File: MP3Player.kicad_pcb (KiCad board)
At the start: 4 copper layers, 40 x 60 mm, 8 parts, among them J1 3.5mm TRRS, SW1 Switch_Tactile_ESwitch, SW2 Switch_Tactile_ESwitch, SW3 Switch_Tactile_ESwitch, SW4 Switch_Tactile_ESwitch, U1 DFR0299, U2 DM-OLED096-636

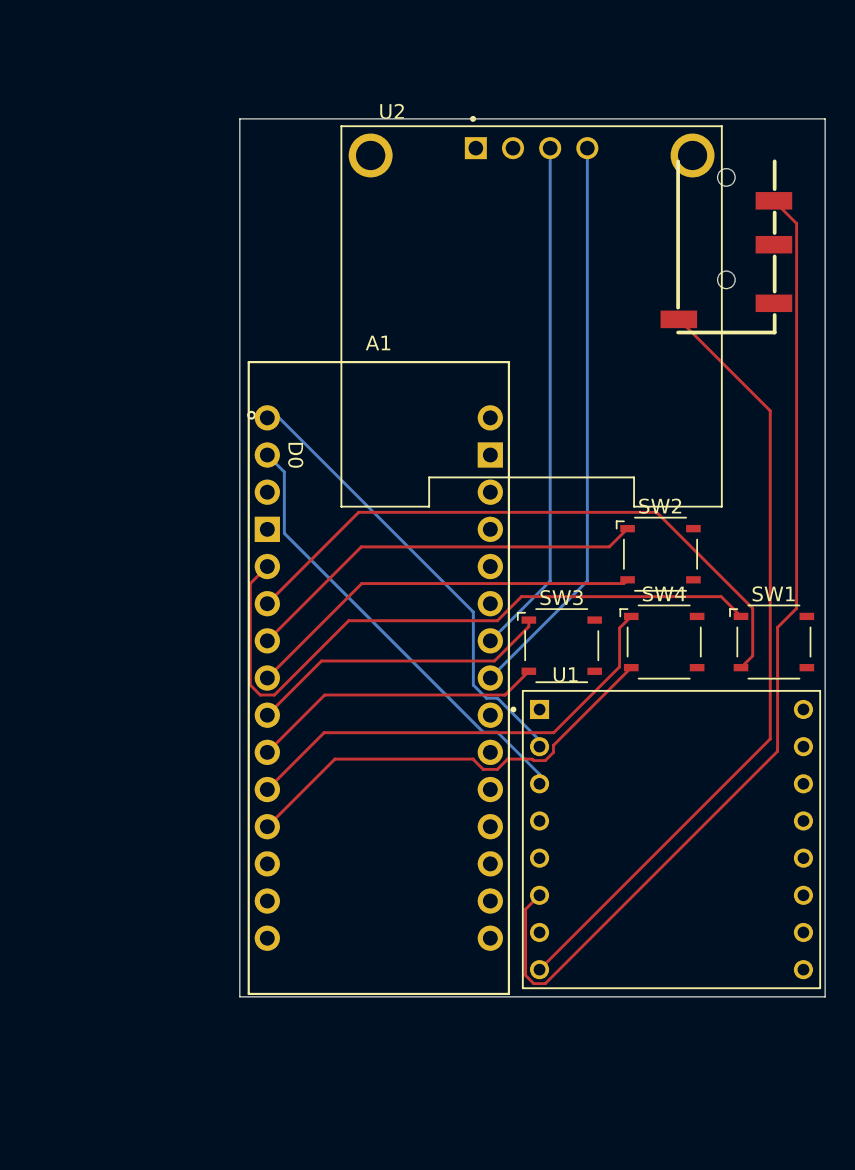
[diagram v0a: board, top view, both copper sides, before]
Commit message: general update
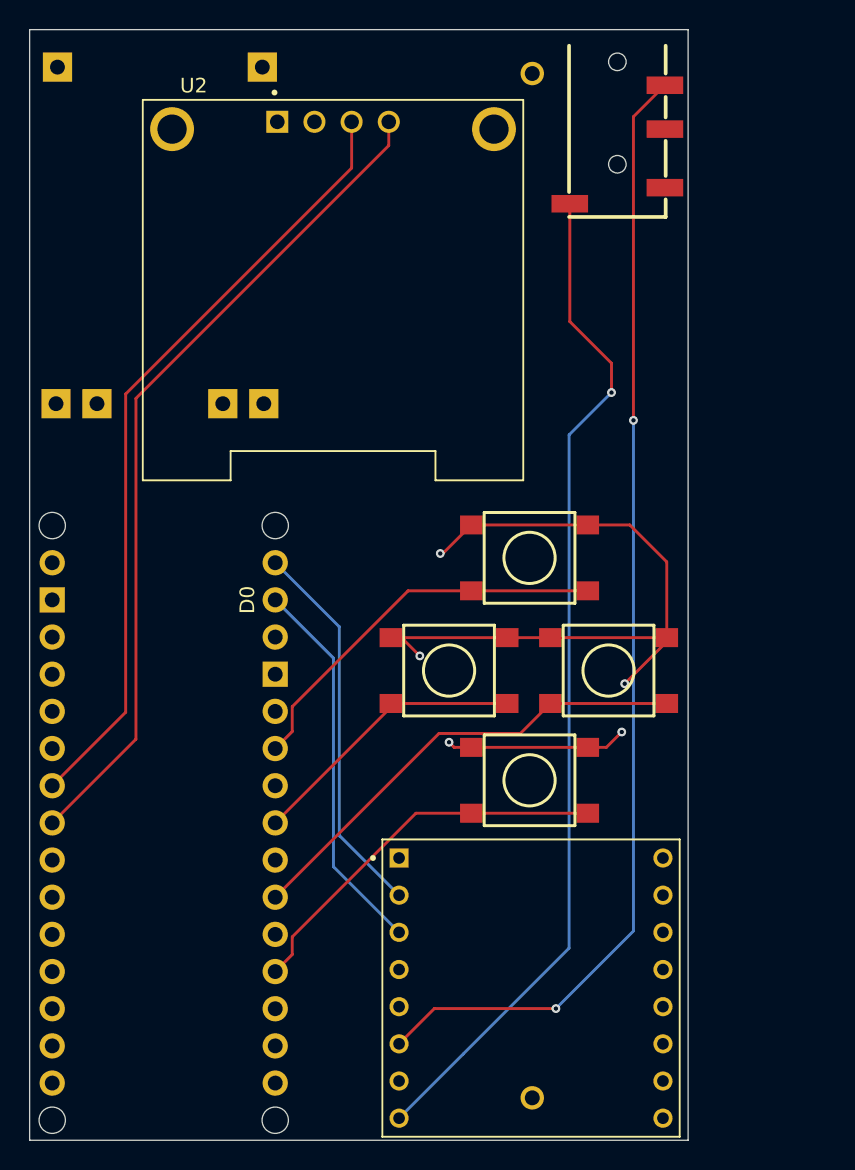
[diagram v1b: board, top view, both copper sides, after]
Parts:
- removed SW1, SW2, SW3, SW4: Switch_Tactile_ESwitch, PCM_fab:Button_ESwitch_TL3315NF100Q_4.5x4.5mm
- added BT2: BH-18650-A1AJ005, JLCImport:BH-18650-A1AJ005, B.Cu at (128.5, 97.4)
- added M1: TP4056Module, Library:TP4056Module, B.Cu at (111.6, 59.5)
- added SWDown1: Switch_Tactile_ESwitch, PCM_SparkFun-Switch:Push_SMD_6.2x6.2mm, F.Cu at (128.3, 110.7)
- added SWLeft1: Switch_Tactile_ESwitch, PCM_SparkFun-Switch:Push_SMD_6.2x6.2mm, F.Cu at (122.8, 103.2)
- added SWRight1: Switch_Tactile_ESwitch, PCM_SparkFun-Switch:Push_SMD_6.2x6.2mm, F.Cu at (133.7, 103.2)
- added SWUp1: Switch_Tactile_ESwitch, PCM_SparkFun-Switch:Push_SMD_6.2x6.2mm, F.Cu at (128.3, 95.5)
- A1: moved to B.Cu
- moved A1 17.7 mm to (103.3, 135.2), turned to 180 degrees
- moved U1 14.0 mm to (128.4, 124.9)
- moved U2 13.7 mm to (114.9, 77.2)
- moved J1 10.9 mm to (134.3, 65.1)
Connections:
- A1 pad D2: Net-(A1-D2_INT0) -> unconnected-(A1-D2_INT0-PadD2)
- A1 pad D4: Net-(A1-PadD4) -> unconnected-(A1-PadD4)
- A1 pad D6: Net-(A1-PadD6) -> unconnected-(A1-PadD6)
- A1 pad D8: Net-(A1-PadD8) -> unconnected-(A1-PadD8)
- A1 pad GND1: GND -> unconnected-(A1-GND-PadGND1)
- A1 pad GND2: Net-(U2-GND) -> Net-(A1-GND-PadGND2)
- A1 pad VIN: unconnected-(A1-PadVIN) -> Net-(M1-OUT+)
- U2 pad 1: Net-(U2-GND) -> GND
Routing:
- net Net-(M1-B+): track 0.00 -> 117.1 mm
- net unconnected-(A1-GND-PadGND1): track 0.00 -> 85.0 mm, vias 0 -> 5
- net Net-(A1-D2_INT0): track 45.7 -> 0.00 mm
- net GND: track 54.0 -> 97.3 mm
- net Net-(M1-B-): track 0.00 -> 35.6 mm
- net Net-(U1-VCC): track 40.4 -> 74.1 mm
- net Net-(A1-PadD8): track 31.3 -> 0.00 mm
- net Net-(A1-PadD4): track 27.8 -> 0.00 mm
- net Net-(U2-GND): track 21.6 -> 0.00 mm
- net Net-(A1-PadD6): track 20.8 -> 0.00 mm
- net Net-(A1-A4/SDA): track 39.0 -> 57.4 mm
- net Net-(A1-A5/SCL): track 35.4 -> 53.8 mm
- net Net-(U1-SPK2): track 53.6 -> 69.7 mm, vias 0 -> 1
- net Net-(A1-D3_INT1): track 42.9 -> 26.8 mm
- net Net-(M1-OUT+): track 0.00 -> 12.9 mm
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- removed copper zone on In1.Cu, net GND
- removed copper zone on In2.Cu, net Net-(U1-VCC)
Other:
- board size 40 x 60 mm -> 45 x 75.9 mm
